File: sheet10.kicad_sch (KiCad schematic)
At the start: 69 parts, among them J1 ISA Bus connector, J10 AT POWER CONNECTOR, J2 ISA Bus connector, J3 ISA Bus connector, J4 ISA Bus connector, J5 ISA Bus connector, J6 ISA Bus connector, J7 ISA Bus connector, J8 ISA Bus connector

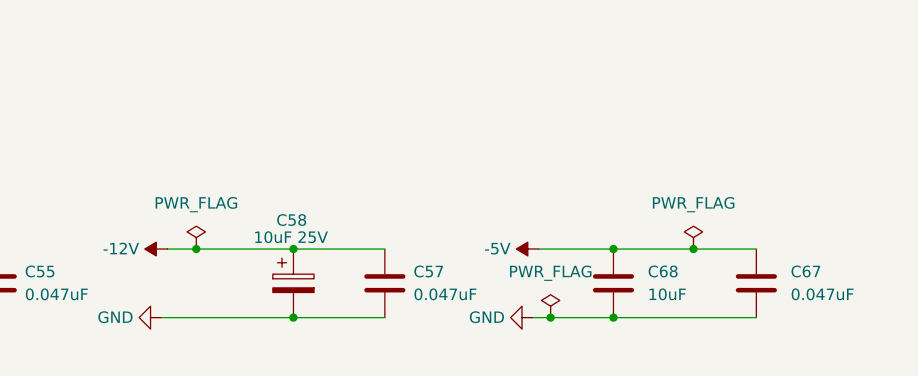
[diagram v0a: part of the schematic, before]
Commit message: Begin tracing
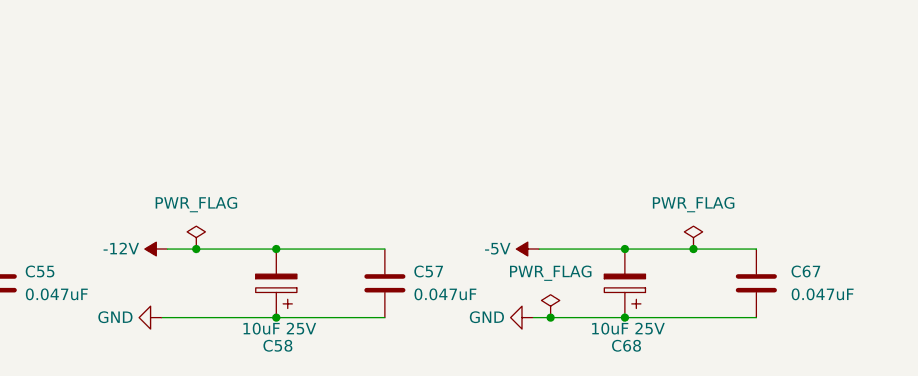
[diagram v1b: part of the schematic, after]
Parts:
- removed C68: 10uF, madXT_early:Cap_unipolar_3pin, symbol Device:C
- added C68: 10uF 25V, madXT_early:cap_tantalum, symbol Device:C_Polarized
- C10, C11, C12, C13, C14, C15, C16, C19, C28, C3, C37, C46, C54, C56, C58, C60, C61, C63: footprint madXT_early:Cap_unipolar_3pin -> madXT_early:cap_tantalum
- C17, C18, C20, C21, C22, C23, C24, C25, C26, C27, C29, C30, C31, C32, C33, C34, C35, C36, C38, C39, C40, C41, C42, C43, C44, C45, C47, C48, C49, C5, C50, C51, C52, C55, C57, C59, C62, C64, C65, C66, C67: footprint Capacitor_THT:C_Disc_D7.0mm_W2.5mm_P5.00mm -> madXT_early:cap_unipolar
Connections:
- net -12V: now also C58.2; no longer C58.1
- net -5V: now also C68.2
- net GND: now also C58.1, C68.1; no longer C58.2
